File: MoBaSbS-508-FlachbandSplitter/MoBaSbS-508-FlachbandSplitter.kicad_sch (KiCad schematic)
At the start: 7 parts, among them J1 Conn_02x05_Odd_Even, J10 1, J11 2, J12 3, J13 4

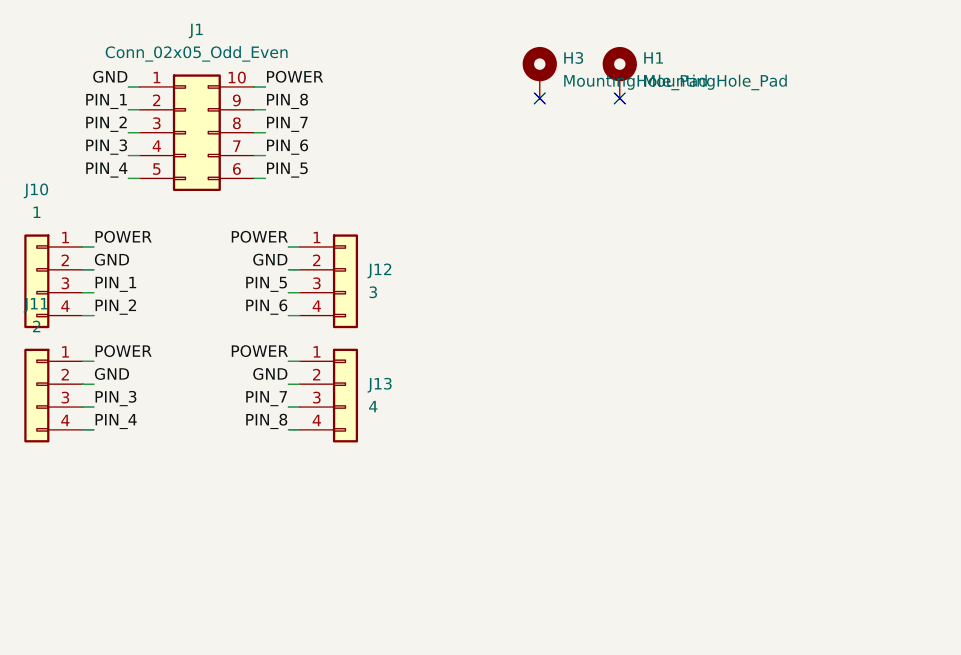
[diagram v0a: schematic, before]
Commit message: Only some finishing touches left
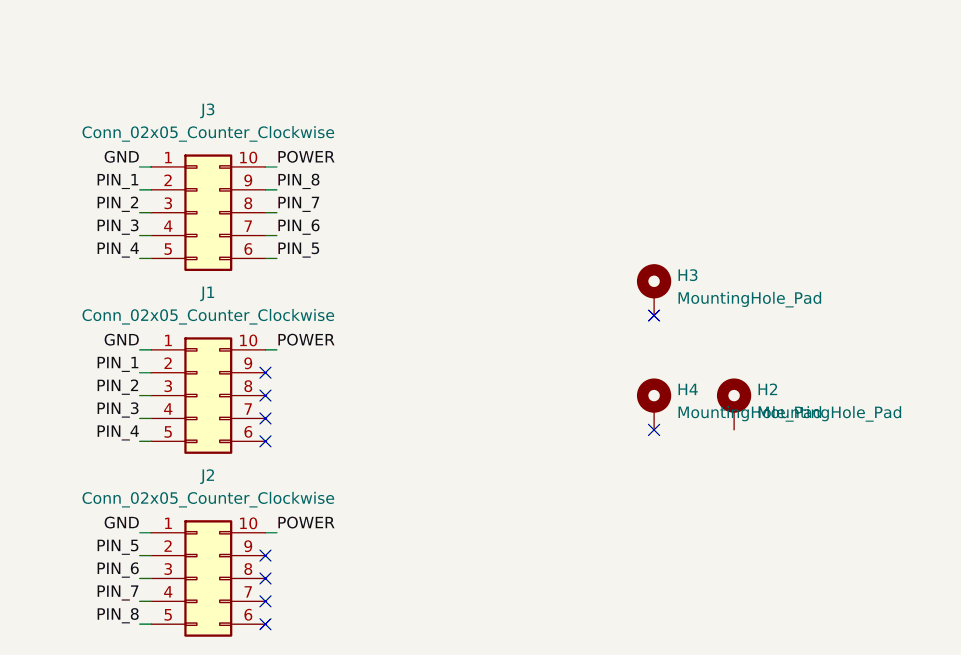
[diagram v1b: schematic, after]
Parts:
- removed H1: MountingHole_Pad, MountingHole:MountingHole_2.7mm_M2.5_DIN965_Pad, symbol Mechanical:MountingHole_Pad
- removed J10: 1, Connector_Molex:Molex_KK-254_AE-6410-04A_1x04_P2.54mm_Vertical, symbol Connector_Generic:Conn_01x04
- removed J11: 2, Connector_Molex:Molex_KK-254_AE-6410-04A_1x04_P2.54mm_Vertical, symbol Connector_Generic:Conn_01x04
- removed J12: 3, Connector_Molex:Molex_KK-254_AE-6410-04A_1x04_P2.54mm_Vertical, symbol Connector_Generic:Conn_01x04
- removed J13: 4, Connector_Molex:Molex_KK-254_AE-6410-04A_1x04_P2.54mm_Vertical, symbol Connector_Generic:Conn_01x04
- added H2, H4: MountingHole_Pad, MountingHole:MountingHole_2.7mm_M2.5_DIN965_Pad, symbol Mechanical:MountingHole_Pad
- added J2, J3: Conn_02x05_Counter_Clockwise, Connector_IDC:IDC-Header_2x05_P2.54mm_Vertical, symbol Connector_Generic:Conn_02x05_Counter_Clockwise
- J1: value Conn_02x05_Odd_Even -> Conn_02x05_Counter_Clockwise
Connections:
- net GND: now also J2.1 (Pin_1), J3.1 (Pin_1)
- net PIN_1: now also J3.2 (Pin_2)
- net PIN_2: now also J3.3 (Pin_3)
- net PIN_3: now also J3.4 (Pin_4)
- net PIN_4: now also J3.5 (Pin_5)
- net PIN_5: now also J2.2 (Pin_2), J3.6 (Pin_6); no longer J1.6 (Pin_6)
- net PIN_6: now also J2.3 (Pin_3), J3.7 (Pin_7); no longer J1.7 (Pin_7)
- net PIN_7: now also J2.4 (Pin_4), J3.8 (Pin_8); no longer J1.8 (Pin_8)
- net PIN_8: now also J2.5 (Pin_5), J3.9 (Pin_9); no longer J1.9 (Pin_9)
- net POWER: now also J2.10 (Pin_10), J3.10 (Pin_10)
- no-connect marks 2 -> 10
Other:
- moved on the sheet: H3
